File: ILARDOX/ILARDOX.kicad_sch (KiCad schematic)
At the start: 18 parts, among them J1 Conn_01x08, J2 Step_Down_Mini, J3 Conn_01x02, J4 Conn_01x02, SW1 SW_Push, SW2 SW_Push, U1 ESP32-S3-WROOM-1, U2 LM358, U3 AMS1117-3.3, U4 24LC256

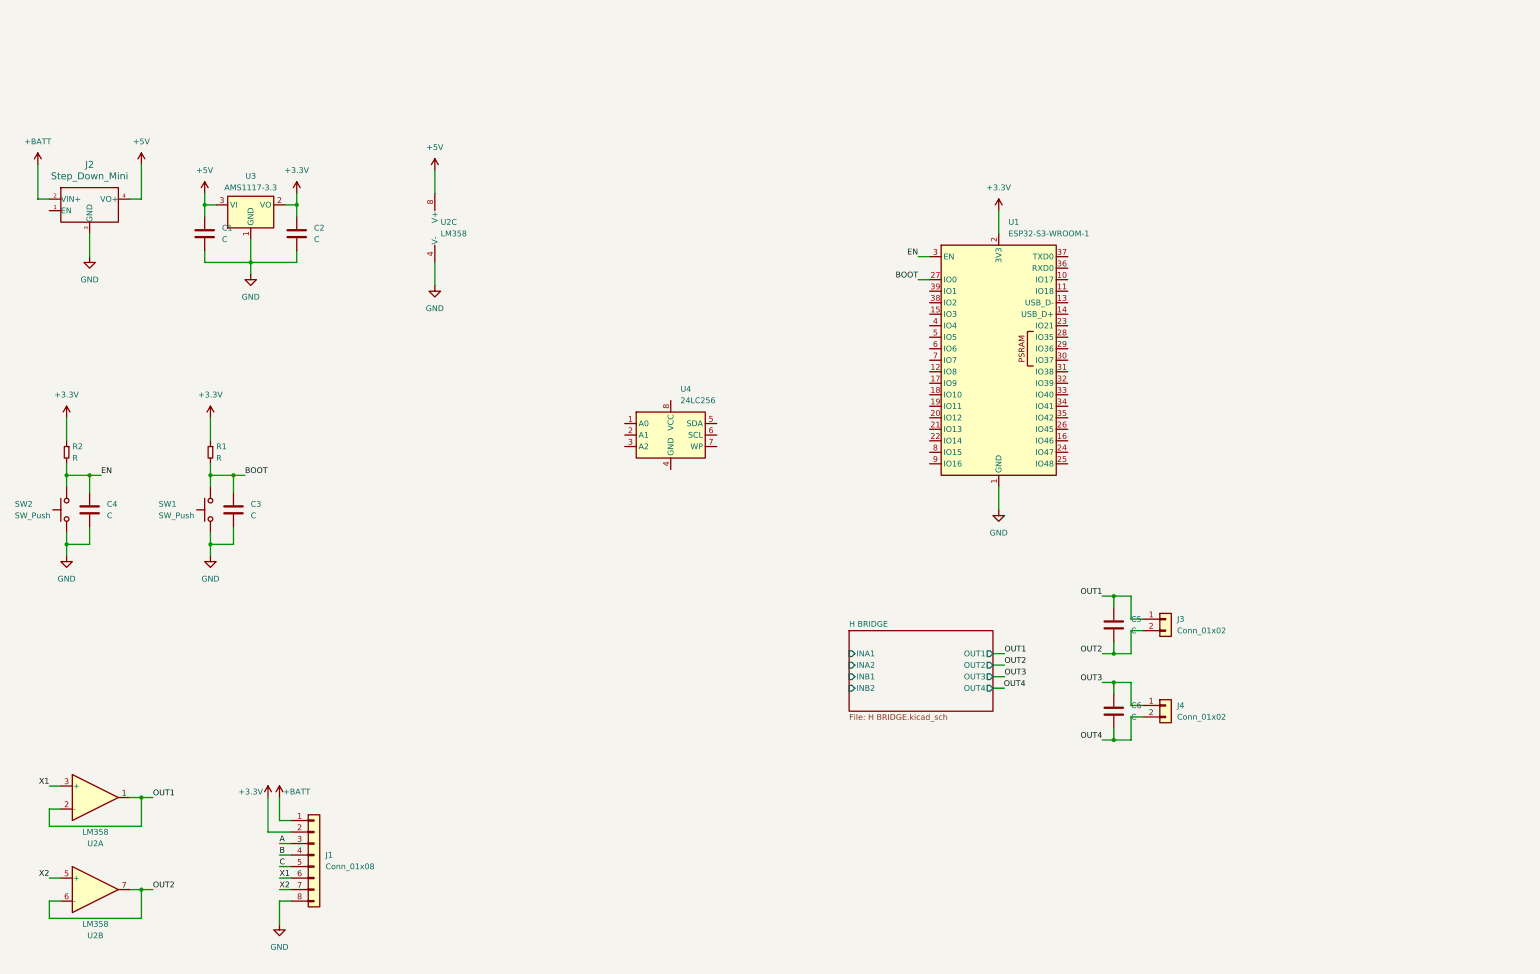
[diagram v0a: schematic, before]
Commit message: new
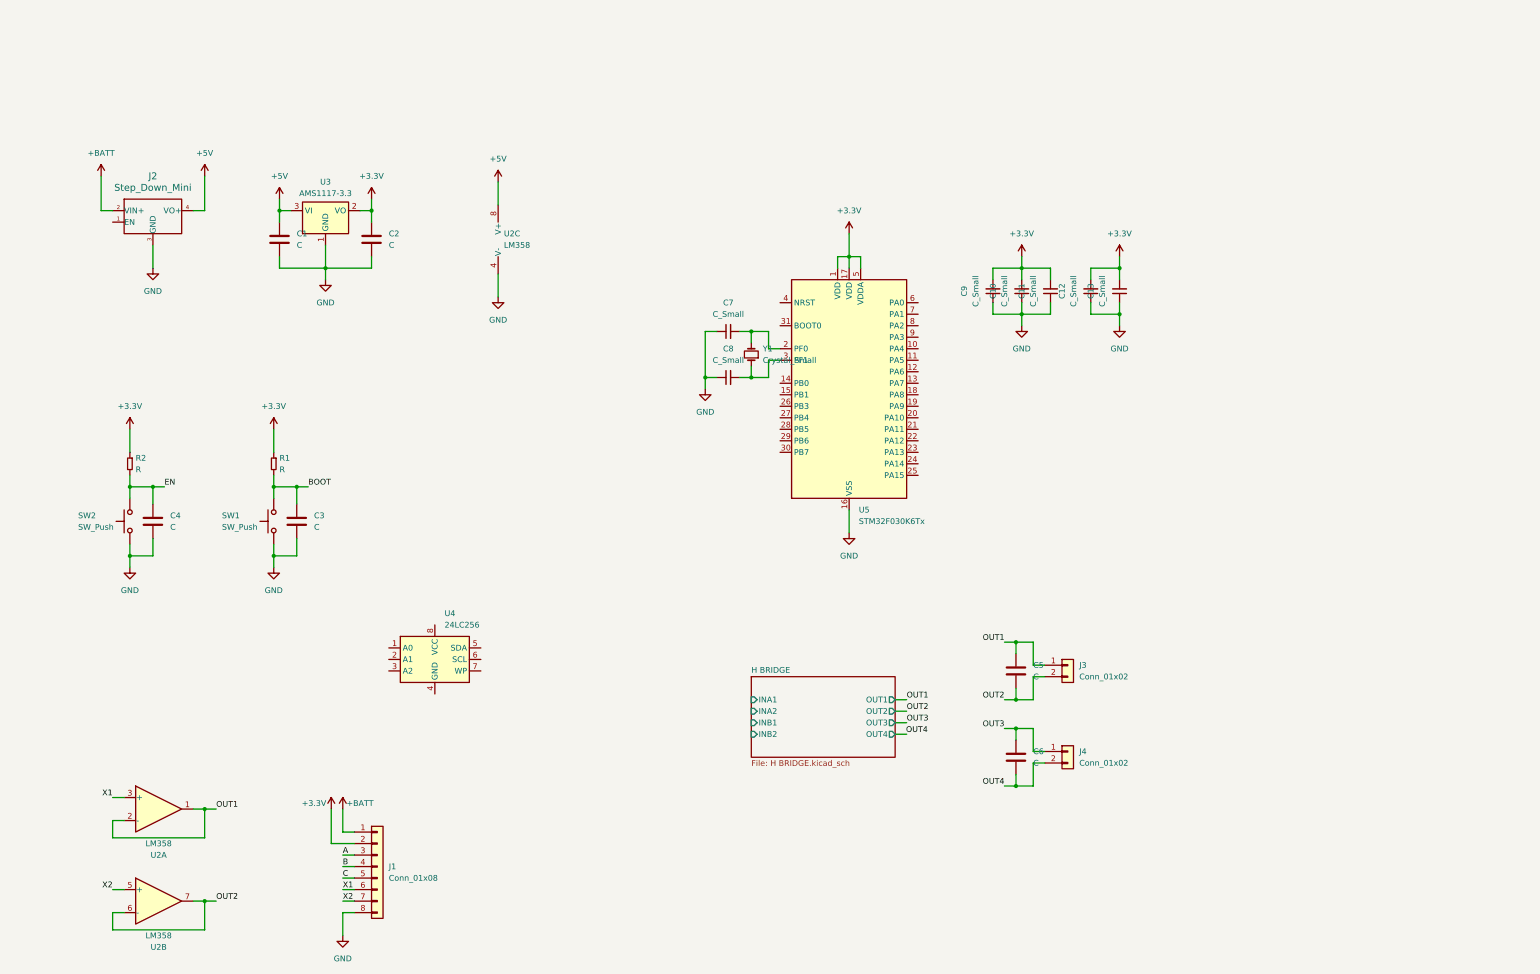
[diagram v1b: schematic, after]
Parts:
- removed U1: ESP32-S3-WROOM-1, RF_Module:ESP32-S3-WROOM-1, symbol RF_Module:ESP32-S3-WROOM-1
- added C10, C11, C12, C13, C7, C8, C9: C_Small, symbol Device:C_Small
- added U5: STM32F030K6Tx, Package_QFP:LQFP-32_7x7mm_P0.8mm, symbol MCU_ST_STM32F0:STM32F030K6Tx
- added Y1: Crystal_Small, symbol Device:Crystal_Small
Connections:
- net +3.3V: now also C10.2, C11.2, C12.2, C13.2, C9.2, U5.1 (VDD), U5.17 (VDD), U5.5 (VDDA)
- net GND: now also C10.1, C11.1, C12.1, C13.1, C7.1, C8.1, C9.1, U5.16 (VSS), U5.32 (VSS)
- new net: C8.2, U5.3 (PF1), Y1.1
- new net: C7.2, U5.2 (PF0), Y1.2
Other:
- moved on the sheet: C1, C2, C3, C4, C5, C6, J1, J2, J3, J4, R1, R2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

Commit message: new
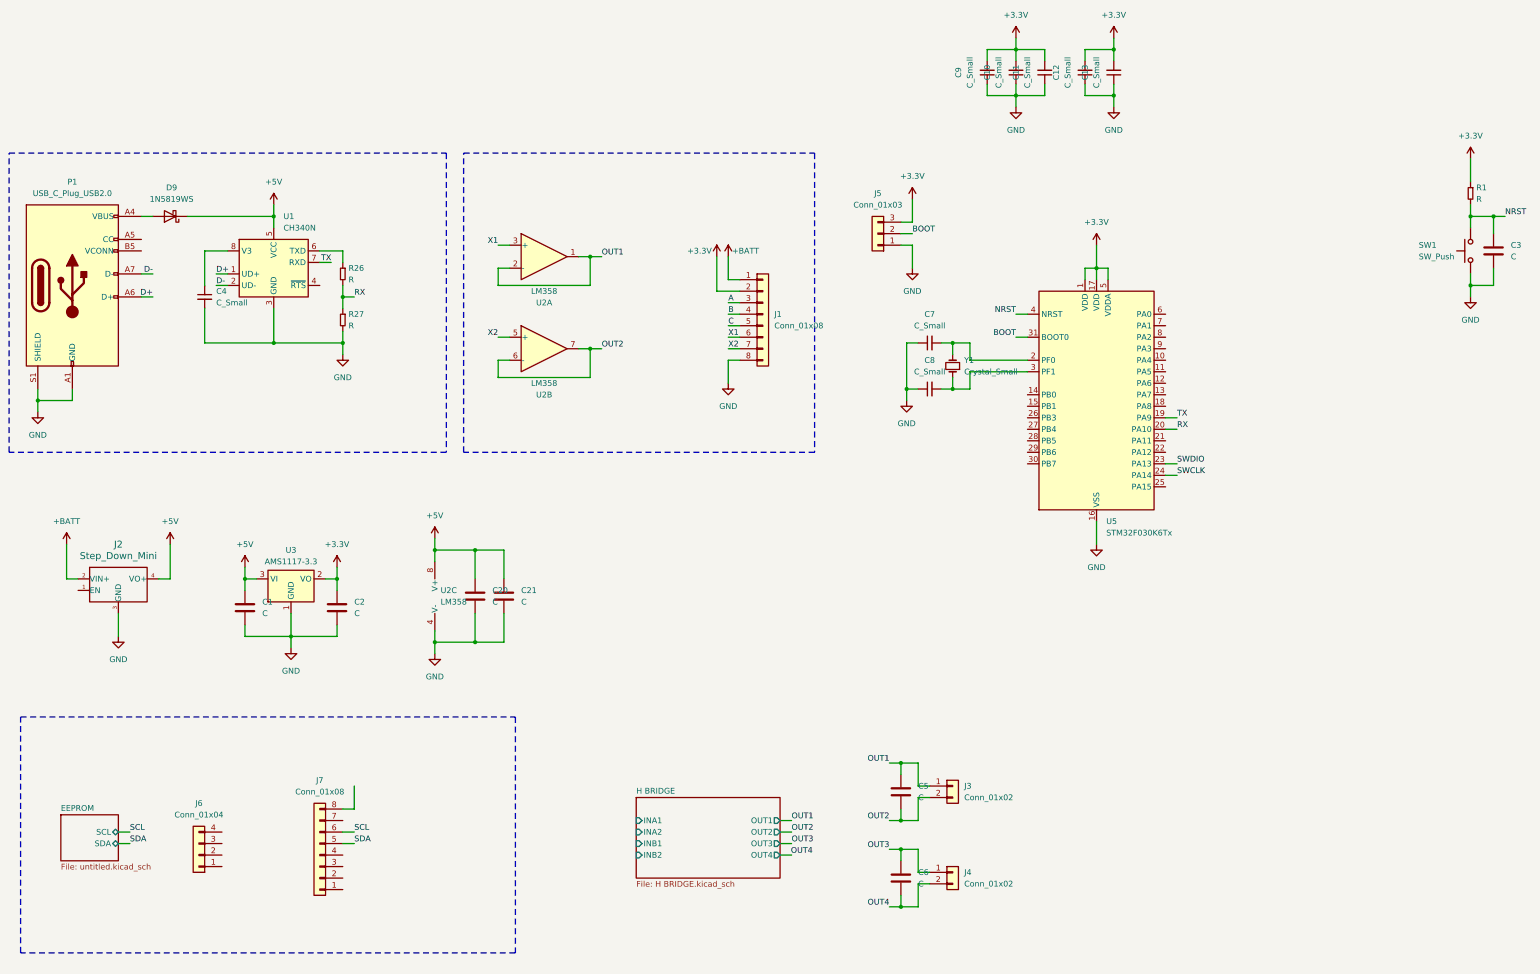
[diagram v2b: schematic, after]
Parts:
- removed C4: C, symbol Device:C
- removed R2: R, symbol EESTN5:R
- removed SW2: SW_Push, symbol Switch:SW_Push
- removed U4: 24LC256, symbol Memory_EEPROM:24LC256
- added C20, C21: C, symbol Device:C
- added C4: C_Small, symbol Device:C_Small
- added D9: 1N5819WS, Diode_SMD:D_SOD-323, symbol Diode:1N5819WS
- added J5: Conn_01x03, symbol Connector_Generic:Conn_01x03
- added J6: Conn_01x04, symbol Connector_Generic:Conn_01x04
- added J7: Conn_01x08, symbol Connector_Generic:Conn_01x08
- added P1: USB_C_Plug_USB2.0, symbol Connector:USB_C_Plug_USB2.0
- added R26, R27: R, symbol EESTN5:R
- added U1: CH340N, Package_SO:SOP-8_3.9x4.9mm_P1.27mm, symbol Interface_USB:CH340N
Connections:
- net +3.3V: now also J5.3 (Pin_3)
- net +5V: now also C20.1, C21.1, D9.1 (K), U1.5 (VCC)
- net BOOT: now also U5.31 (BOOT0), J5.2 (Pin_2); no longer C3.1, R1.2, SW1.2
- net GND: now also C20.2, C21.2, C4.2, J5.1 (Pin_1), P1.A1 (GND), P1.A12 (GND), P1.B1 (GND), P1.B12 (GND), P1.S1 (SHIELD), R27.2, U1.3 (GND)
- net TX: now reaches U5.19 (PA9)
- net TX: now also U1.7 (RXD)
- net RX: now reaches U5.20 (PA10)
- net RX: now also R26.2, R27.1
- net SWDIO: now reaches U5.23 (PA13)
- net SWCLK: now reaches U5.24 (PA14)
- net NRST: now reaches U5.4 (NRST)
- net NRST: now also C3.1, R1.2, SW1.2
- new net: D9.2 (A), P1.A4 (VBUS), P1.A9 (VBUS), P1.B4 (VBUS), P1.B9 (VBUS)
- new net: C4.1, U1.8 (V3)
- new net: R26.1, U1.6 (TXD)
- new net D+: P1.A6 (D+), U1.1 (UD+)
- new net D-: P1.A7 (D-), U1.2 (UD-)
- new net SCL: J7.6 (Pin_6)
- new net SDA: J7.5 (Pin_5)
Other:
- added sheet EEPROM (untitled.kicad_sch)
- moved on the sheet: C1, C10, C11, C12, C13, C2, C3, C5, C6, C7, C8, C9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
